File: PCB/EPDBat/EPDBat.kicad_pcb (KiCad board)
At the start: 2 copper layers, 70 x 70 mm, 51 parts, among them J1 Conn_01x26, J10 JST-PH-SM3-TB, J4 Conn_01x02, J5 TC2030-USB-NL-DS, J7 USB-C-Socket-V, Q1 BSS138, Q2 CJ2301, Q3 C179347, U1 TP4054, U2 ME6211C33M5G-N, U4 ESP32-S3-MINI-1

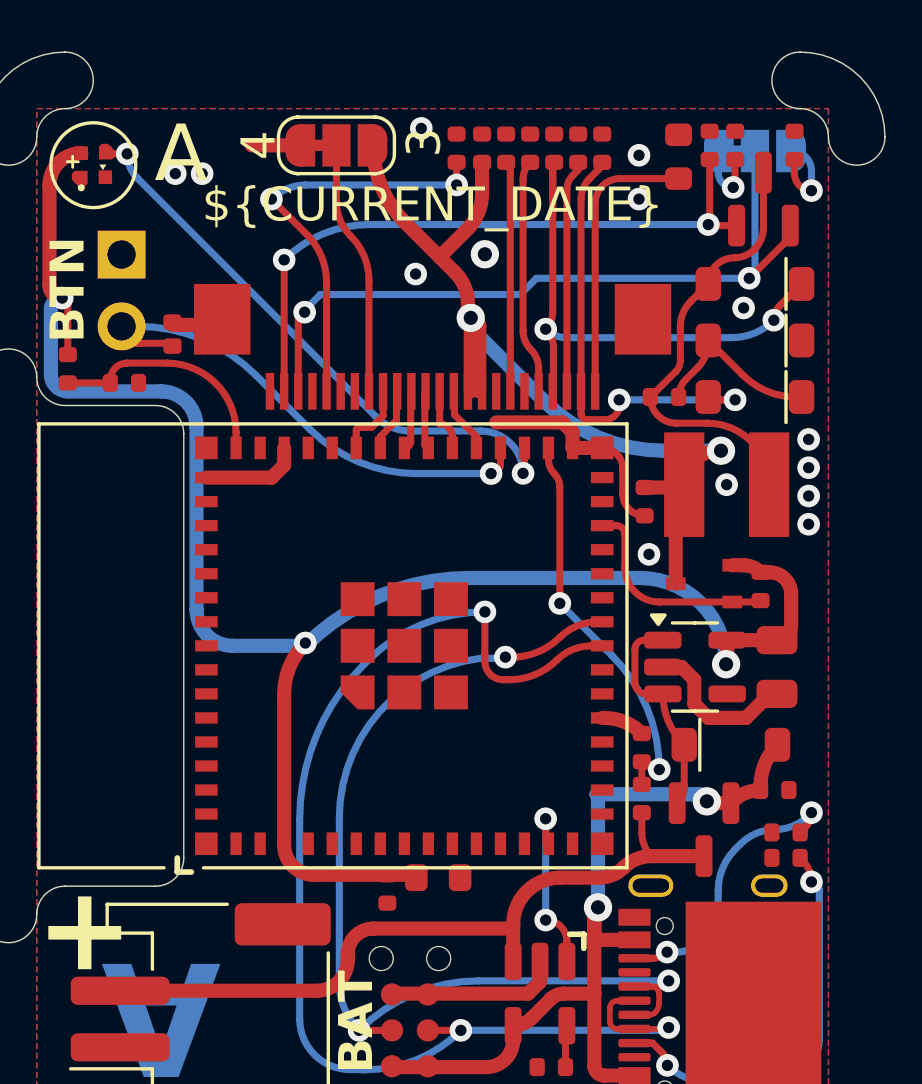
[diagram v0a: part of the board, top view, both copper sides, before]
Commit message: New connectors
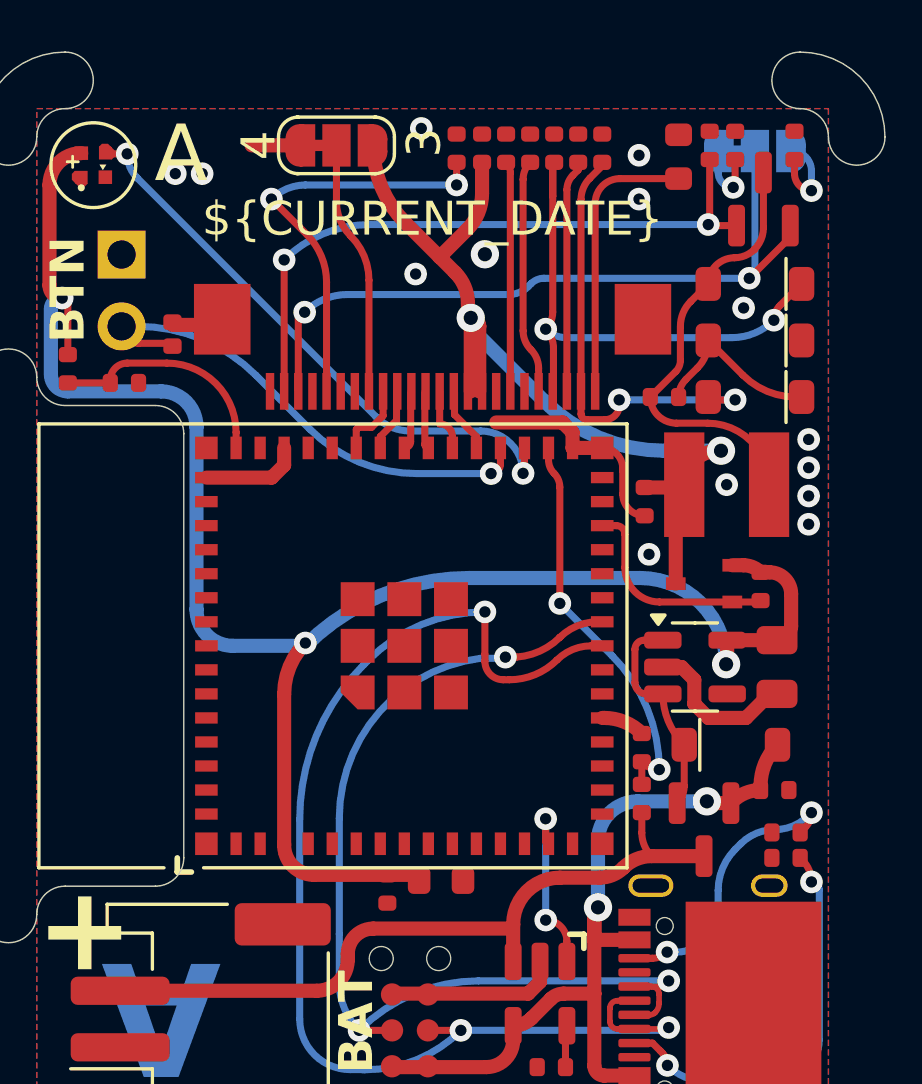
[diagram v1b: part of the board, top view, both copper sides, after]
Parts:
- moved C5 0.14 mm to (100.3, 98.3)
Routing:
- net VBUS: track 30.0 -> 29.0 mm
